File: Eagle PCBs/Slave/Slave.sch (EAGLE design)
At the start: 8 parts, among them Q1 TIP120

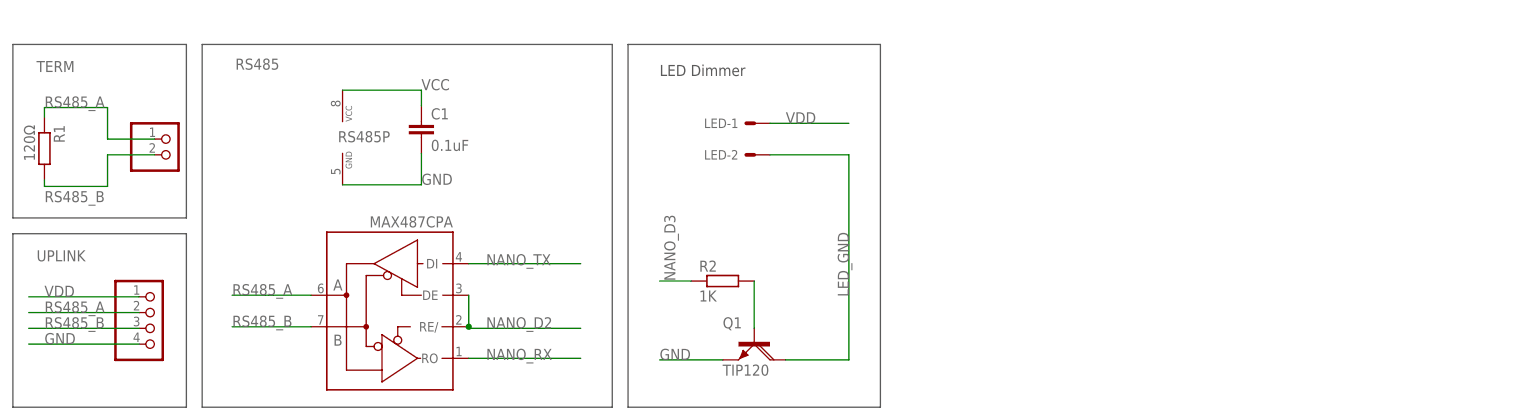
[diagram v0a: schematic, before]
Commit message: New slave PCB
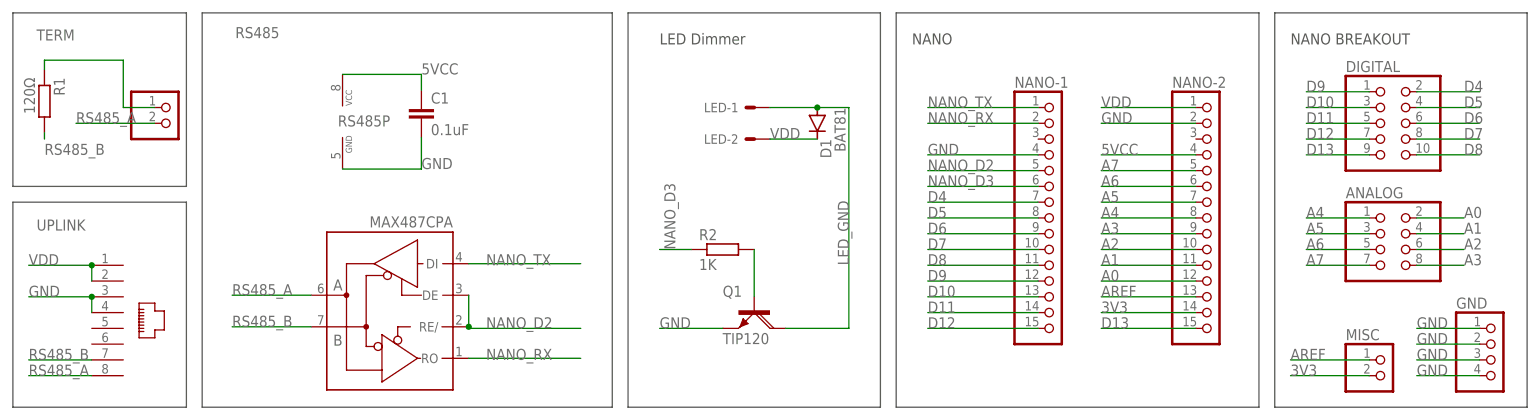
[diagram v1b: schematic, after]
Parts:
- added ANALOG: (no value), pinhead:PINHD-2X4
- added D1: BAT81, diode:BAT81
- added DIGITAL: (no value), pinhead:PINHD-2X5
- added GND: (no value), pinhead:PINHD-1X4
- added MISC: (no value), pinhead:PINHD-1X2
- added NANO-1, NANO-2: (no value), pinhead:PINHD-1X15
- R1, R2: device rcl:R-EU_0207/10 -> rcl:R-EU_0204/7
- UPLINK: value (none) -> RJ45-8P8C; device pinhead:PINHD-1X4 -> A10 Library:RJ45-8P8C
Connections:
- net N$2 renamed LED_PWM
- removed net VCC: C1.1, RS485P.VCC
- new net 3V3: MISC.2, NANO-2.14
- new net 5VCC: C1.1, NANO-2.4, RS485P.VCC
- new net A0: ANALOG.2, NANO-2.12
- new net A1: ANALOG.4, NANO-2.11
- new net A2: ANALOG.6, NANO-2.10
- new net A3: ANALOG.8, NANO-2.9
- new net A4: ANALOG.1, NANO-2.8
- new net A5: ANALOG.3, NANO-2.7
- new net A6: ANALOG.5, NANO-2.6
- new net A7: ANALOG.7, NANO-2.5
- new net AREF: MISC.1, NANO-2.13
- new net D10: DIGITAL.3, NANO-1.13
- new net D11: DIGITAL.5, NANO-1.14
- new net D12: DIGITAL.7, NANO-1.15
- new net D13: DIGITAL.9, NANO-2.15
- new net D4: DIGITAL.2, NANO-1.7
- new net D5: DIGITAL.4, NANO-1.8
- new net D6: DIGITAL.6, NANO-1.9
- new net D7: DIGITAL.8, NANO-1.10
- new net D8: DIGITAL.10, NANO-1.11
- new net D9: DIGITAL.1, NANO-1.12
- new net TERM: R1.1, TERM.1
- net GND: now also GND.1, GND.2, GND.3, GND.4, NANO-1.4, NANO-2.2, UPLINK.3
- net LED_GND: now also D1.A, LED-1.S; no longer LED-2.S
- net NANO_D2: now also NANO-1.5
- net NANO_D3: now also NANO-1.6
- net NANO_RX: now also NANO-1.2
- net NANO_TX: now also NANO-1.1
- net RS485_A: now also TERM.2, UPLINK.8; no longer R1.1, TERM.1, UPLINK.2
- net RS485_B: now also UPLINK.7; no longer TERM.2, UPLINK.3
- net VDD: now also D1.C, LED-2.S, NANO-2.1, UPLINK.2; no longer LED-1.S
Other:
- note added: "NANO"
- note added: "NANO BREAKOUT"
- moved on the sheet: C1, LED-1, LED-2, Q1, R1, R2, RS485P, TERM
